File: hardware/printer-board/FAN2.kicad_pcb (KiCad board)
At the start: 2 copper layers, 8 parts, among them J1 TO FAN2, Q1 D882

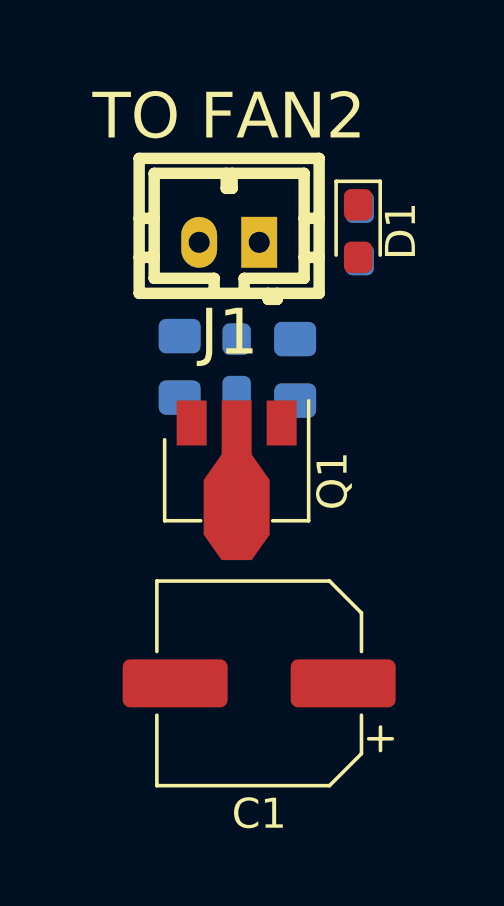
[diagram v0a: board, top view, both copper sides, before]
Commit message: update,
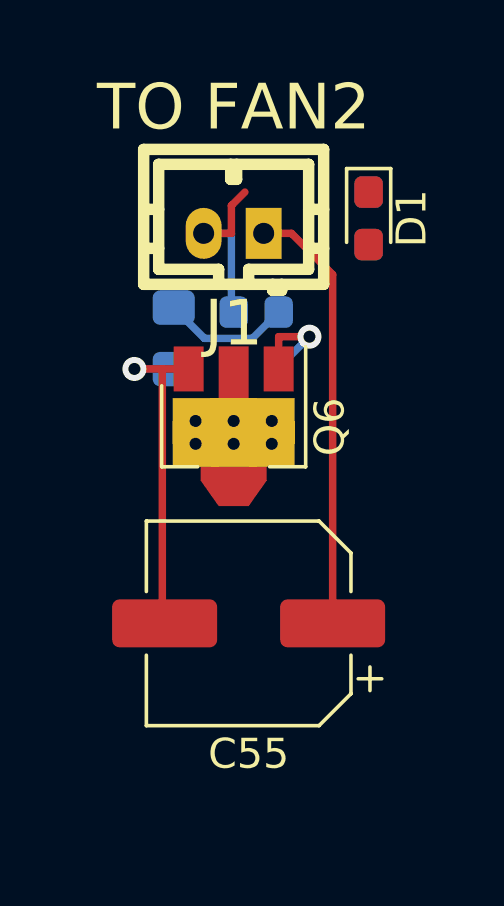
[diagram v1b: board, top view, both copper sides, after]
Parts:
- removed C1: CP100uf,16V, Capacitor_SMD:CP_Elec_6.3x5.3
- removed Q1: D882, Package_TO_SOT_SMD:SOT-89-3
- removed R1: R182,0603, Resistor_SMD:R_0603_1608Metric_Pad1.05x0.95mm_HandSolder
- removed R2: R100,0603, Resistor_SMD:R_0603_1608Metric_Pad1.05x0.95mm_HandSolder
- removed R4: R104,0805, Resistor_SMD:R_0805_2012Metric_Pad1.15x1.40mm_HandSolder
- added C55: CP100uf,16V, Capacitor_SMD:CP_Elec_6.3x5.3, F.Cu at (7.50, 16.5)
- added Q6: D882, footprint-lib:SOT-89-3,thermal_vias, F.Cu at (7.00, 9.50)
- added R48: R182,0603, Resistor_SMD:R_0603_1608Metric_Pad1.05x0.95mm_HandSolder, B.Cu at (11.5, 3.00)
- added R49: R100,0603, Resistor_SMD:R_0603_1608Metric_Pad1.05x0.95mm_HandSolder, B.Cu at (7.00, 7.00)
- added R86: R104,0805, Resistor_SMD:R_0805_2012Metric_Pad1.15x1.40mm_HandSolder, B.Cu at (5.00, 7.00)
- R3: footprint Resistor_SMD:R_0805_2012Metric_Pad1.15x1.40mm_HandSolder -> Resistor_SMD:R_0603_1608Metric_Pad1.05x0.95mm_HandSolder
- moved R3 1.19 mm to (8.50, 7.00)
- moved D1 0.55 mm to (11.5, 3.00)
- moved J1 0.34 mm to (7.00, 3.50)
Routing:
- net +12V: track 0.00 -> 14.5 mm
- net GND: track 0.00 -> 11.6 mm, vias 0 -> 1
- net Net-(Q6-Pad2): track 0.00 -> 9.94 mm
- net Net-(D1-Pad1): track 0.00 -> 6.07 mm
- net /FAN_EN: track 0.00 -> 4.29 mm
- net Net-(Q6-Pad1): track 0.00 -> 3.51 mm, vias 0 -> 1
